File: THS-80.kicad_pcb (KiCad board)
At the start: 4 copper layers, 101.6 x 101.6 mm, 102 parts, among them J1 USB_B_Micro, J10 CTC Header, J2 RC80 Bus, J3 RC80 Expansion, J4 IDE, J5 JTAG, J6 PMOD, J7 PIO Header, J8 Port B, J9 Port A, Q1 IRLML6402, Q2 IRLML6402, SW1 Reset, SW2 SW_DIP_x06, U1 MAX40203AUK, U2 DS1813R-5+T&R, U3 EPM7064STC100, U4 Z84C0010AEG, U5 IS62C5128BL-45TLI, U6 SST39SF040, U7 Z84C2010AEG, U8 Z84C4310AEG, U9 Z84C3010AEG, X1 CFPS-72 50mhz

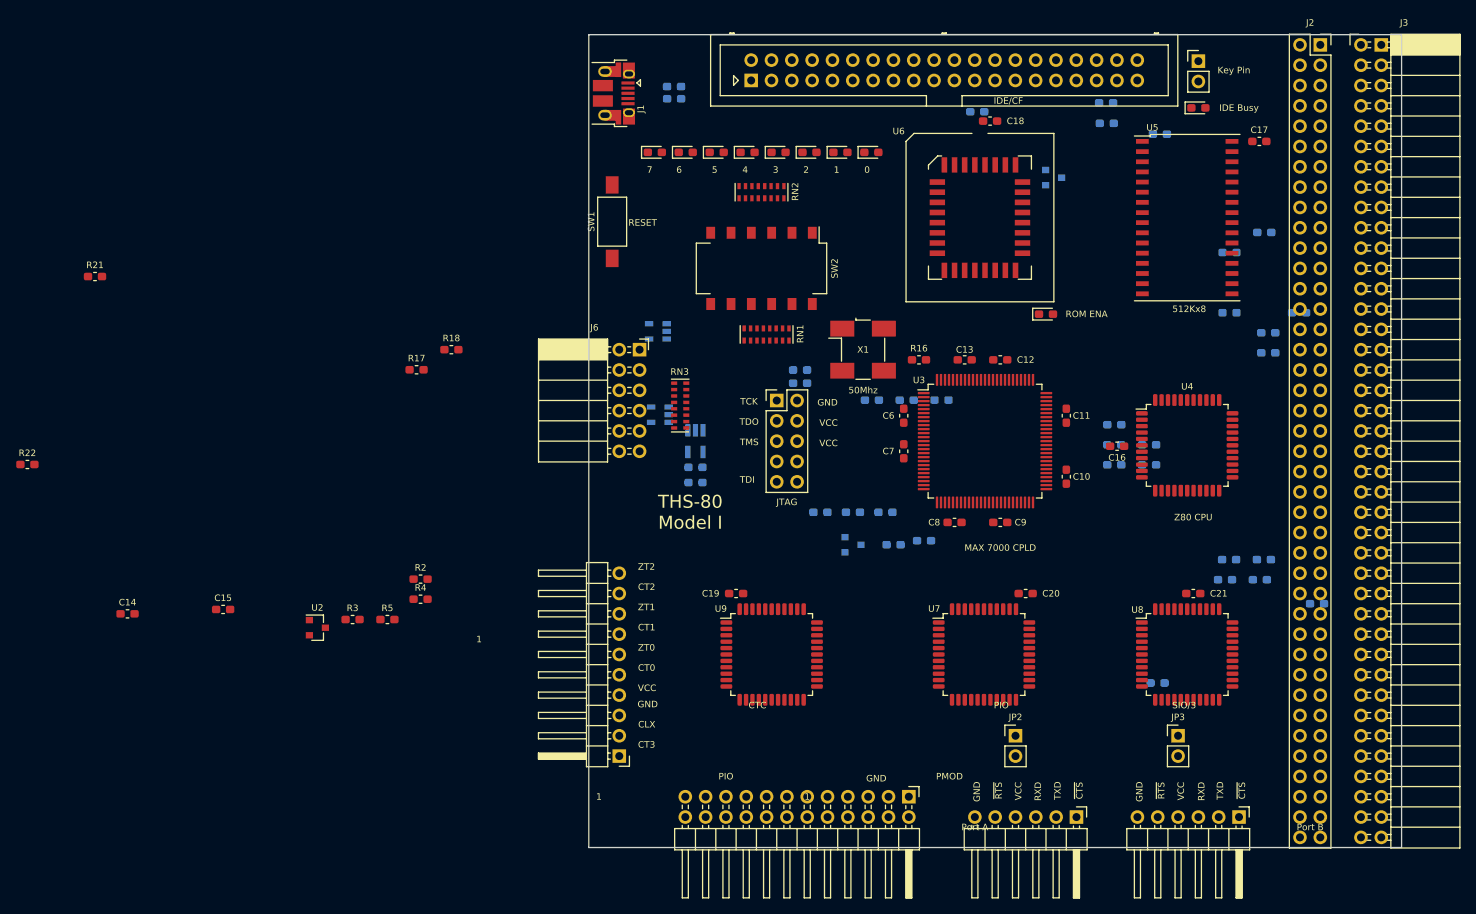
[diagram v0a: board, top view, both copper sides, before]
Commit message: started routing
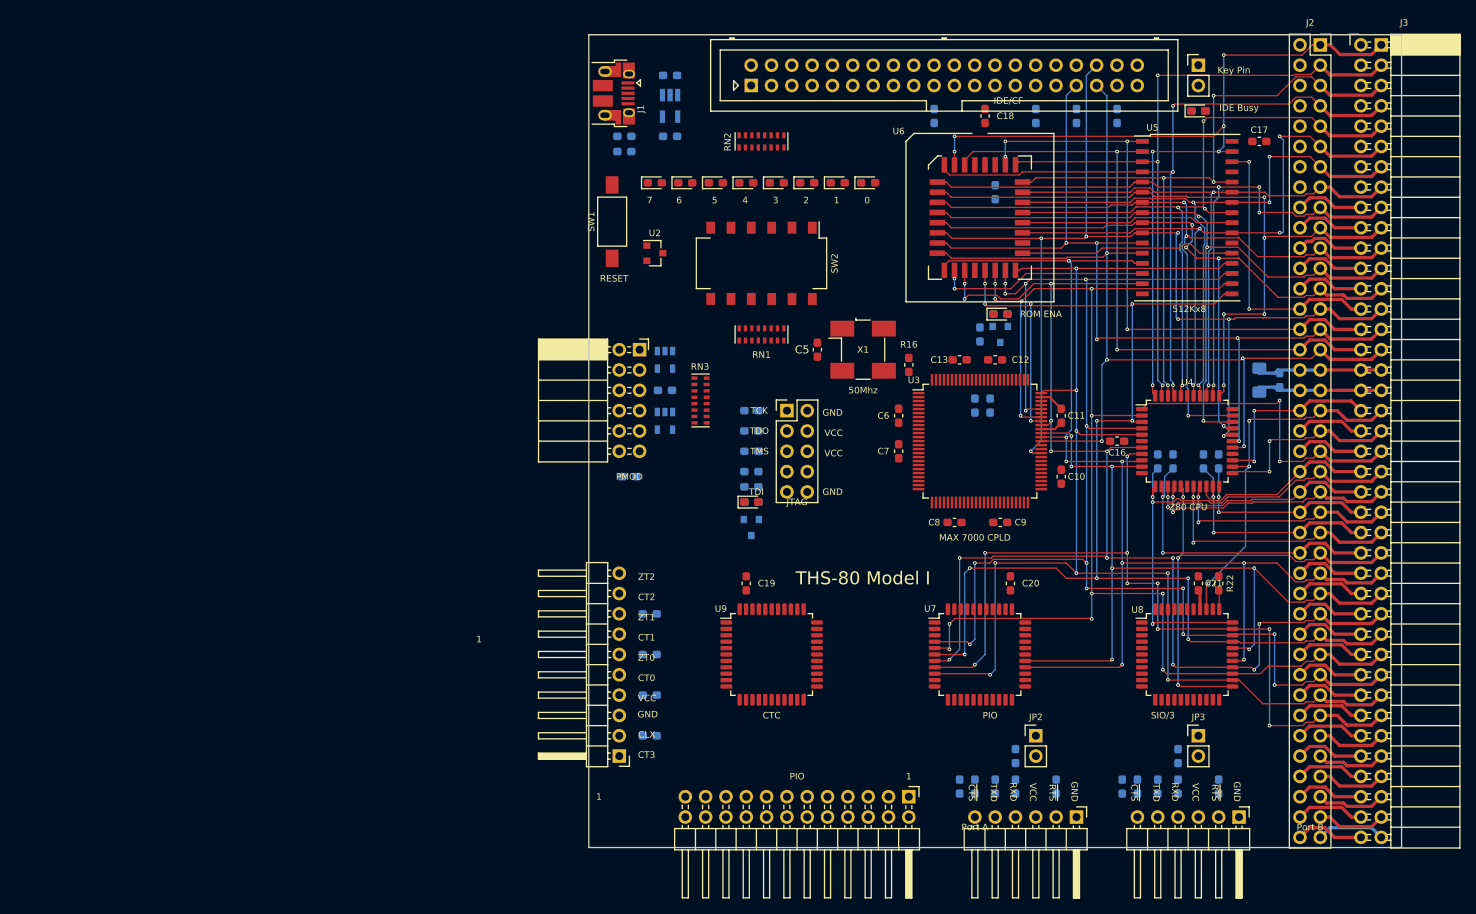
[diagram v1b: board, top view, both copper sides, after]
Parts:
- added C22: 100uF, Capacitor_SMD:C_1206_3216Metric_Pad1.42x1.75mm_HandSolder, B.Cu at (185.4, 74.9)
- added C23: 100nF, Capacitor_SMD:C_0603_1608Metric_Pad1.05x0.95mm_HandSolder, B.Cu at (188.0, 74.9)
- C14, C15, R17, R18, R2, R21, R3, R4, R5: moved to B.Cu
- C2: value 100nF -> 2.2nF
- C3: value 1uF -> .33uF
- C5, D13: moved to F.Cu
- moved R22 149.7 mm to (180.3, 100.3), turned to 270 degrees
- moved R21 113.0 mm to (152.4, 51.4), turned to 90 degrees
- moved R5 105.8 mm to (180.3, 85.1), turned to 270 degrees
- moved R3 104.4 mm to (174.6, 85.1), turned to 270 degrees
- moved R4 99.4 mm to (178.4, 85.1), turned to 270 degrees
- moved R2 93.3 mm to (172.7, 85.1), turned to 270 degrees
- moved R35 79.9 mm to (109.2, 119.4), turned to 180 degrees
- moved R17 71.8 mm to (151.8, 78.1), turned to 270 degrees
- moved R37 67.7 mm to (109.2, 109.2), turned to 180 degrees
- moved R15 67.4 mm to (121.9, 90.2)
- moved R36 67.2 mm to (109.2, 114.3), turned to 180 degrees
- moved R14 66.8 mm to (121.9, 88.3)
- moved R18 65.8 mm to (149.9, 78.1), turned to 270 degrees
- moved R12 65.8 mm to (121.9, 81.3)
- moved C14 65.0 mm to (106.7, 87.0)
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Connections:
- C3 pad 1: VCC -> Net-(C3-Pad1)
- C4 pad 1: Net-(C4-Pad1) -> VCC
- D12 pad 1: /CPLD/R7 -> /CPLD/R4
- D12 pad 3: /CPLD/R6 -> /CPLD/R5
- D12 pad 4: /CPLD/R5 -> /CPLD/R6
- D12 pad 5: /CPLD/R4 -> /CPLD/R7
- J1 pad 1: Net-(J1-Pad1) -> Net-(C3-Pad1)
- J4 pad 20: Net-(C4-Pad1) -> Net-(J4-Pad20)
- J5 pad 6: VCC -> (no net)
- JP1 pad 1: Net-(C4-Pad1) -> Net-(J4-Pad20)
- RN2 pad 1: Net-(D11-Pad2) -> Net-(D4-Pad2)
- RN2 pad 2: Net-(D10-Pad2) -> Net-(D5-Pad2)
- RN2 pad 3: Net-(D9-Pad2) -> Net-(D6-Pad2)
- RN2 pad 4: Net-(D8-Pad2) -> Net-(D7-Pad2)
- RN2 pad 5: Net-(D7-Pad2) -> Net-(D8-Pad2)
- RN2 pad 6: Net-(D6-Pad2) -> Net-(D9-Pad2)
- RN2 pad 7: Net-(D5-Pad2) -> Net-(D10-Pad2)
- RN2 pad 8: Net-(D4-Pad2) -> Net-(D11-Pad2)
- U1 pad 1: Net-(J1-Pad1) -> Net-(C3-Pad1)
- U1 pad 3: Net-(J1-Pad1) -> Net-(C3-Pad1)
- U3 pad 45: (no net) -> /~WAIT
- U3 pad 92: /A16 -> (no net)
- U3 pad 93: /A17 -> (no net)
- U3 pad 94: /A18 -> (no net)
- U3 pad 96: (no net) -> /A16
- U3 pad 97: (no net) -> /A17
- U3 pad 98: (no net) -> /A18
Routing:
- net /D5: track 0.00 -> 175.8 mm, vias 0 -> 14
- net /D4: track 0.00 -> 169.9 mm, vias 0 -> 12
- net /D3: track 0.00 -> 167.7 mm, vias 0 -> 12
- net /D6: track 0.00 -> 164.5 mm, vias 0 -> 8
- net /D2: track 0.00 -> 162.8 mm, vias 0 -> 13
- net /D0: track 0.00 -> 149.9 mm, vias 0 -> 8
- net /A2: track 0.00 -> 135.6 mm, vias 0 -> 7
- net /D7: track 0.00 -> 133.5 mm, vias 0 -> 9
- net /D1: track 0.00 -> 127.6 mm, vias 0 -> 9
- net /A0: track 0.00 -> 127.4 mm, vias 0 -> 5
- net /A15: track 0.00 -> 111.9 mm, vias 0 -> 7
- net /A1: track 0.00 -> 109.3 mm, vias 0 -> 5
- net /A12: track 0.00 -> 94.1 mm, vias 0 -> 3
- net /A5: track 0.00 -> 91.7 mm, vias 0 -> 3
- net /A4: track 0.00 -> 88.7 mm, vias 0 -> 3
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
